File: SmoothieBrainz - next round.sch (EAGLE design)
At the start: 232 parts, among them IC1 LPC1769, IC7 74LVC1G04, Q1 BSL207SP, Q2 12MHz, SW1 SW_TACT_4P_B, SW3 SW_TACT_4P_B, T1 BC817, U3 USD-SOCKETUSD, X1 MSTBA2, X14 USBPTH, X2 GMSTBA2, X3 GMSTBA4, X4 1751248, X5 1751248, X6 1751248, X7 1751248

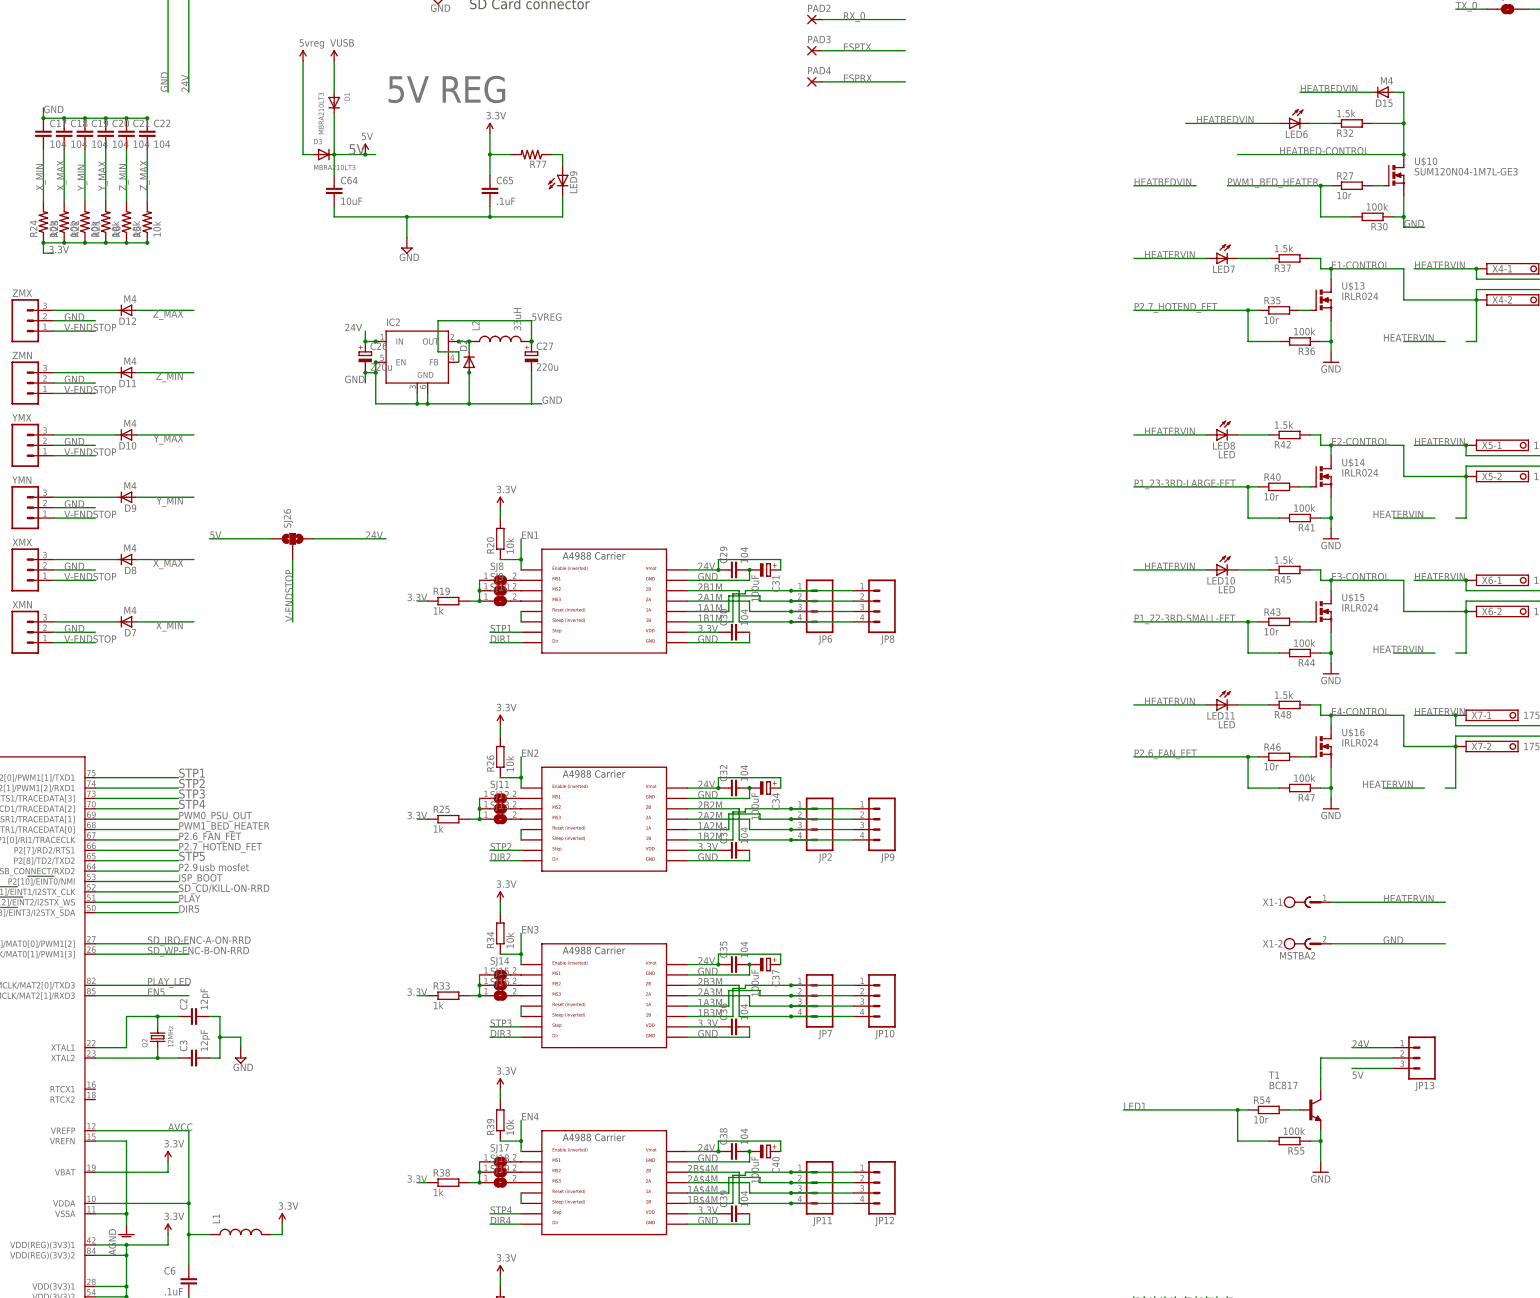
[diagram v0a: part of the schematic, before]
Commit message: rev2 initial ready
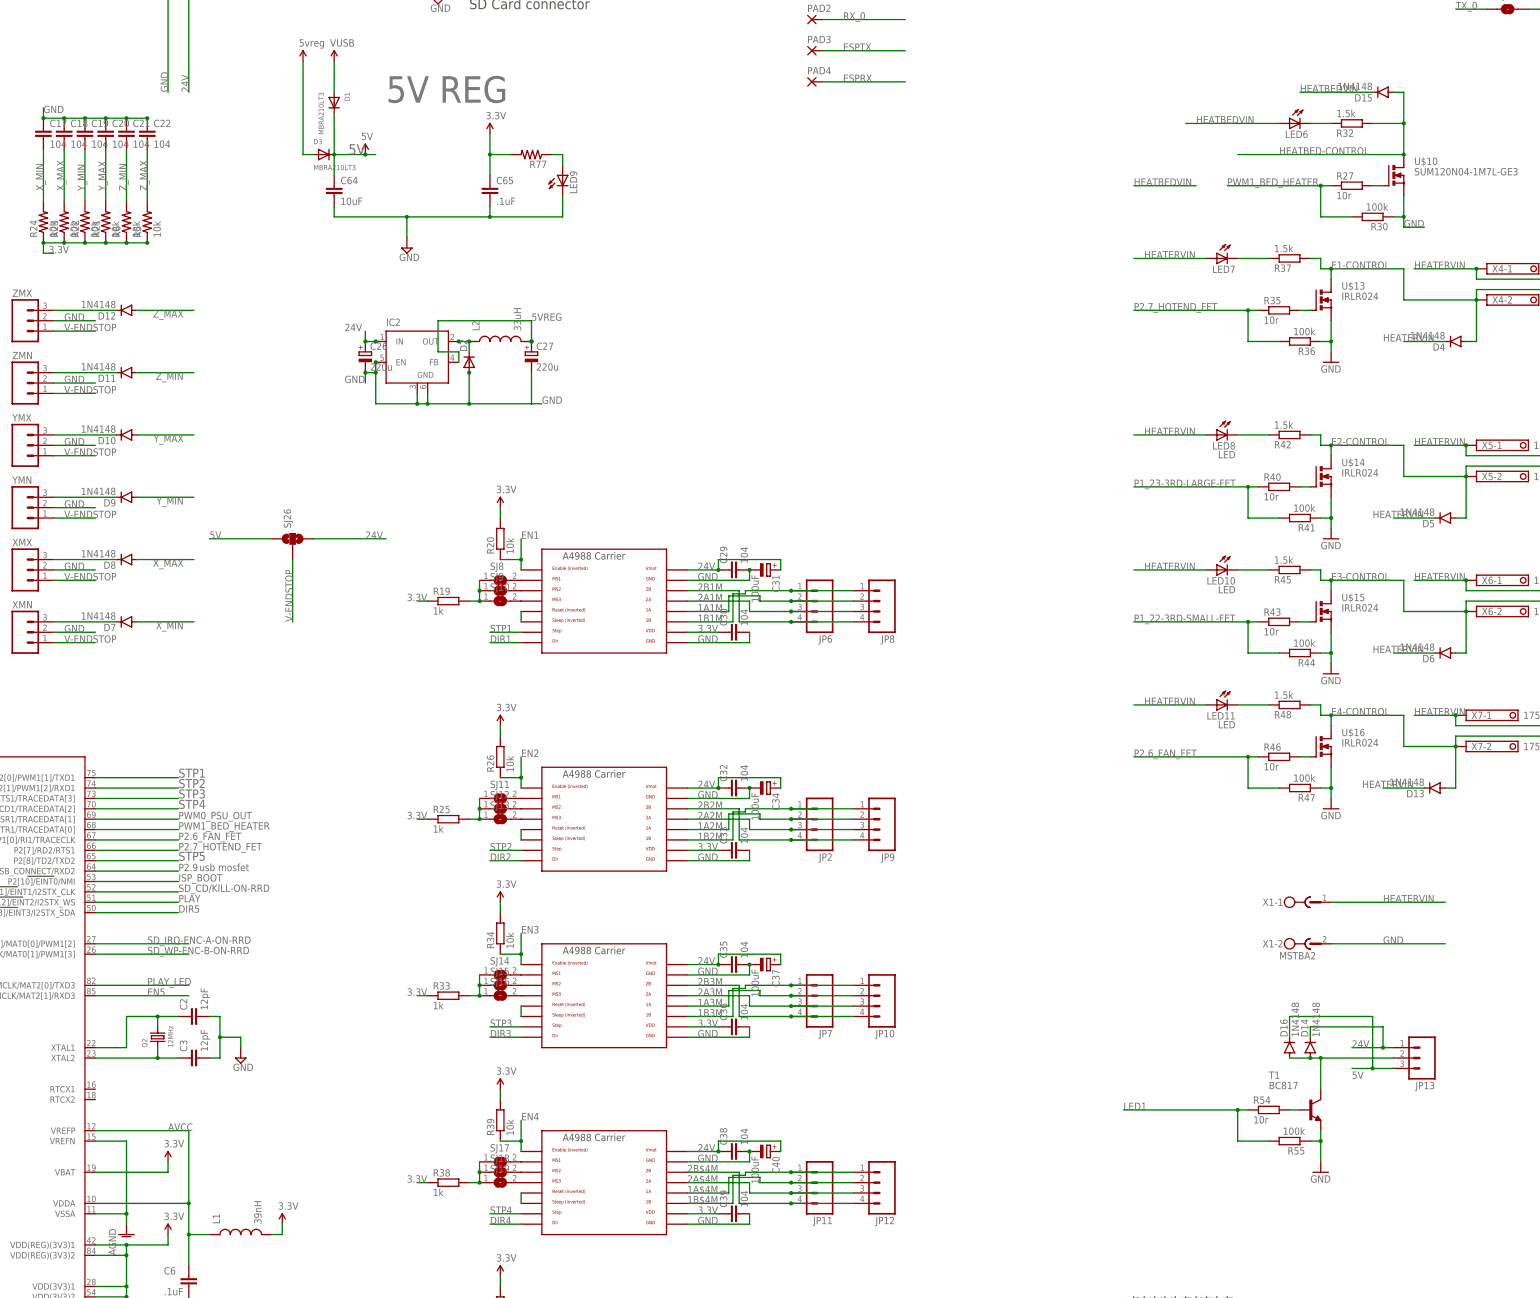
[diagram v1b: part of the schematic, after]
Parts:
- added D13, D14, D16, D4, D5, D6: 1N4148, SparkFun-DiscreteSemi:DIODEBAS16
- D10, D11, D12, D15, D7, D8, D9: value M4 -> 1N4148; device semicon-smd-ipc:D-SOD-87 -> SparkFun-DiscreteSemi:DIODEBAS16
- L1: value (none) -> 39nH
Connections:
- net 24V: now also D14.C
- net 5V: now also D16.C
- net E1-CONTROL: now also D4.A
- net E2-CONTROL: now also D5.A
- net E3-CONTROL: now also D6.A
- net E4-CONTROL: now also D13.A
- net HEATERVIN: now also D13.C, D4.C, D5.C, D6.C
- net N$56: now also D14.A, D16.A
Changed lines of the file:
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@@
 <part name="SUPPLY3" library="supply2" deviceset="GND" device=""/>
 <part name="C7" library="resistor" deviceset="C-EU" device="C0603" value="10uF"/>
-<part name="L1" library="SparkFun" deviceset="INDUCTOR" device="0603"/>
+<part name="L1" library="SparkFun" deviceset="INDUCTOR" device="0603" value="39nH"/>
 <part name="C6" library="rcl" deviceset="C-EU" device="C0603" value=".1uF"/>
 <part name="R14" library="resistor" deviceset="R-US_" device="R0603" value="10K"/>
@@
 <part name="EXP1" library="con-3m" deviceset="2510-" device=""/>
 <part name="EXP2" library="con-3m" deviceset="2510-" device=""/>
-<part name="D7" library="semicon-smd-ipc" deviceset="D-" device="SOD-87" value="M4"/>
-<part name="D8" library="semicon-smd-ipc" deviceset="D-" device="SOD-87" value="M4"/>
-<part name="D9" library="semicon-smd-ipc" deviceset="D-" device="SOD-87" value="M4"/>
-<part name="D10" library="semicon-smd-ipc" deviceset="D-" device="SOD-87" value="M4"/>
-<part name="D11" library="semicon-smd-ipc" deviceset="D-" device="SOD-87" value="M4"/>
-<part name="D12" library="semicon-smd-ipc" deviceset="D-" device="SOD-87" value="M4"/>
+<part name="D7" library="SparkFun-DiscreteSemi" deviceset="DIODE" device="BAS16" value="1N4148"/>
+<part name="D8" library="SparkFun-DiscreteSemi" deviceset="DIODE" device="BAS16" value="1N4148"/>
+<part name="D9" library="SparkFun-DiscreteSemi" deviceset="DIODE" device="BAS16" value="1N4148"/>
+<part name="D10" library="SparkFun-DiscreteSemi" deviceset="DIODE" device="BAS16" value="1N4148"/>
+<part name="D11" library="SparkFun-DiscreteSemi" deviceset="DIODE" device="BAS16" value="1N4148"/>
+<part name="D12" library="SparkFun-DiscreteSemi" deviceset="DIODE" device="BAS16" value="1N4148"/>
 <part name="R5" library="adafruit" deviceset="R-US_" device="R0603" value="10k"/>
 <part name="R6" library="adafruit" deviceset="R-US_" device="R0603" value="10k"/>
@@
 <part name="JP13" library="SparkFun-Connectors" deviceset="M03" device="LOCK"/>
 <part name="X1" library="con-phoenix-508" deviceset="MSTBA2" device=""/>
-<part name="D15" library="semicon-smd-ipc" deviceset="D-" device="SOD-87" value="M4"/>
+<part name="D15" library="SparkFun-DiscreteSemi" deviceset="DIODE" device="BAS16" value="1N4148"/>
 <part name="JP17" library="SparkFun-Connectors" deviceset="M08" device="LOCK"/>
 <part name="AGND4" library="supply1" deviceset="AGND" device=""/>
@@
 <part name="JP22" library="SparkFun-Connectors" deviceset="M02" device="LOCK"/>
 <part name="JP23" library="SparkFun-Connectors" deviceset="M02" device="LOCK"/>
+<part name="D4" library="SparkFun-DiscreteSemi" deviceset="DIODE" device="BAS16" value="1N4148"/>
+<part name="D5" library="SparkFun-DiscreteSemi" deviceset="DIODE" device="BAS16" value="1N4148"/>
+<part name="D6" library="SparkFun-DiscreteSemi" deviceset="DIODE" device="BAS16" value="1N4148"/>
+<part name="D13" library="SparkFun-DiscreteSemi" deviceset="DIODE" device="BAS16" value="1N4148"/>
+<part name="D14" library="SparkFun-DiscreteSemi" deviceset="DIODE" device="BAS16" value="1N4148"/>
+<part name="D16" library="SparkFun-DiscreteSemi" deviceset="DIODE" device="BAS16" value="1N4148"/>
 </parts>
 <sheets>
@@
 <instance part="JP22" gate="G$1" x="607.06" y="264.16" rot="R180"/>
 <instance part="JP23" gate="G$1" x="607.06" y="231.14" rot="R180"/>
+<instance part="D4" gate="G$1" x="551.18" y="325.12" rot="R180"/>
+<instance part="D5" gate="G$1" x="548.64" y="281.94" rot="R180"/>
+<instance part="D6" gate="G$1" x="548.64" y="248.92" rot="R180"/>
+<instance part="D13" gate="G$1" x="546.1" y="215.9" rot="R180"/>
+<instance part="D14" gate="G$1" x="515.62" y="152.4" rot="R90"/>
+<instance part="D16" gate="G$1" x="510.54" y="152.4" rot="R90"/>
 </instances>
 <busses>
@@
 <pinref part="GND4" gate="1" pin="GND"/>
 <pinref part="T1" gate="G$1" pin="E"/>
-<wire x1="518.16" y1="124.46" x2="518.16" y2="129.54" width="0.1524" layer="91"/>
 <pinref part="R55" gate="G$1" pin="1"/>
+<wire x1="518.16" y1="124.46" x2="518.16" y2="129.54" width="0.1524" layer="91"/>
 <wire x1="518.16" y1="129.54" x2="518.16" y2="132.08" width="0.1524" layer="91"/>
 <wire x1="515.62" y1="129.54" x2="518.16" y2="129.54" width="0.1524" layer="91"/>
@@
 <segment>
 <pinref part="JP13" gate="G$1" pin="3"/>
-<wire x1="535.94" y1="147.32" x2="525.78" y2="147.32" width="0.1524" layer="91"/>
+<wire x1="535.94" y1="147.32" x2="530.86" y2="147.32" width="0.1524" layer="91"/>
 <label x="525.78" y="144.78" size="1.778" layer="95"/>
+<pinref part="D16" gate="G$1" pin="C"/>
+<wire x1="530.86" y1="147.32" x2="525.78" y2="147.32" width="0.1524" layer="91"/>
+<wire x1="510.54" y1="154.94" x2="510.54" y2="160.02" width="0.1524" layer="91"/>
+<wire x1="510.54" y1="160.02" x2="530.86" y2="160.02" width="0.1524" layer="91"/>
+<wire x1="530.86" y1="160.02" x2="530.86" y2="147.32" width="0.1524" layer="91"/>
+<junction x="530.86" y="147.32"/>
 </segment>
 <segment>
@@
 <segment>
 <pinref part="JP13" gate="G$1" pin="1"/>
-<wire x1="535.94" y1="152.4" x2="525.78" y2="152.4" width="0.1524" layer="91"/>
 <label x="525.78" y="152.4" size="1.778" layer="95"/>
+<wire x1="535.94" y1="152.4" x2="533.4" y2="152.4" width="0.1524" layer="91"/>
+<pinref part="D14" gate="G$1" pin="C"/>
+<wire x1="533.4" y1="152.4" x2="525.78" y2="152.4" width="0.1524" layer="91"/>
+<wire x1="515.62" y1="154.94" x2="515.62" y2="157.48" width="0.1524" layer="91"/>
+<wire x1="515.62" y1="157.48" x2="533.4" y2="157.48" width="0.1524" layer="91"/>
+<wire x1="533.4" y1="157.48" x2="533.4" y2="152.4" width="0.1524" layer="91"/>
+<junction x="533.4" y="152.4"/>
 </segment>
 <segment>
@@
 <wire x1="599.44" y1="337.82" x2="556.26" y2="337.82" width="0.1524" layer="91"/>
 <wire x1="556.26" y1="337.82" x2="556.26" y2="335.28" width="0.1524" layer="91"/>
+<pinref part="D4" gate="G$1" pin="A"/>
 </segment>
 </net>
@@
 <wire x1="548.64" y1="325.12" x2="538.48" y2="325.12" width="0.1524" layer="91"/>
 <label x="533.4" y="325.12" size="1.778" layer="95"/>
+<pinref part="D4" gate="G$1" pin="C"/>
 </segment>
 <segment>
 <wire x1="546.1" y1="281.94" x2="535.94" y2="281.94" width="0.1524" layer="91"/>
 <label x="530.86" y="281.94" size="1.778" layer="95"/>
+<pinref part="D5" gate="G$1" pin="C"/>
 </segment>
 <segment>
 <wire x1="546.1" y1="248.92" x2="535.94" y2="248.92" width="0.1524" layer="91"/>
 <label x="530.86" y="248.92" size="1.778" layer="95"/>
+<pinref part="D6" gate="G$1" pin="C"/>
 </segment>
 <segment>
 <wire x1="543.56" y1="215.9" x2="533.4" y2="215.9" width="0.1524" layer="91"/>
 <label x="528.32" y="215.9" size="1.778" layer="95"/>
+<pinref part="D13" gate="G$1" pin="C"/>
 </segment>
 <segment>
@@
 <segment>
 <pinref part="T1" gate="G$1" pin="C"/>
-<wire x1="518.16" y1="142.24" x2="518.16" y2="144.78" width="0.1524" layer="91"/>
 <pinref part="JP13" gate="G$1" pin="2"/>
-<wire x1="518.16" y1="144.78" x2="518.16" y2="147.32" width="0.1524" layer="91"/>
+<wire x1="518.16" y1="142.24" x2="518.16" y2="149.86" width="0.1524" layer="91"/>
 <wire x1="535.94" y1="149.86" x2="518.16" y2="149.86" width="0.1524" layer="91"/>
-<wire x1="518.16" y1="149.86" x2="518.16" y2="147.32" width="0.1524" layer="91"/>
+<pinref part="D14" gate="G$1" pin="A"/>
+<wire x1="518.16" y1="149.86" x2="515.62" y2="149.86" width="0.1524" layer="91"/>
+<junction x="518.16" y="149.86"/>
+<pinref part="D16" gate="G$1" pin="A"/>
+<wire x1="515.62" y1="149.86" x2="510.54" y2="149.86" width="0.1524" layer="91"/>
+<junction x="515.62" y="149.86"/>
 </segment>
 </net>
@@
 <junction x="553.72" y="292.1"/>
 <wire x1="553.72" y1="294.64" x2="553.72" y2="292.1" width="0.1524" layer="91"/>
+<pinref part="D5" gate="G$1" pin="A"/>
 </segment>
 </net>
@@
 <junction x="553.72" y="259.08"/>
 <wire x1="553.72" y1="261.62" x2="553.72" y2="259.08" width="0.1524" layer="91"/>
+<pinref part="D6" gate="G$1" pin="A"/>
 </segment>
 </net>
@@
 <junction x="551.18" y="226.06"/>
 <wire x1="551.18" y1="228.6" x2="551.18" y2="226.06" width="0.1524" layer="91"/>
+<pinref part="D13" gate="G$1" pin="A"/>
 </segment>
 </net>
